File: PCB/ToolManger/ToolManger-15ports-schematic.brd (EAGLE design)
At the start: 187.9 x 114.9 mm, 52 parts, among them IC3 4049N, IC4 4049N, IC5 4049N

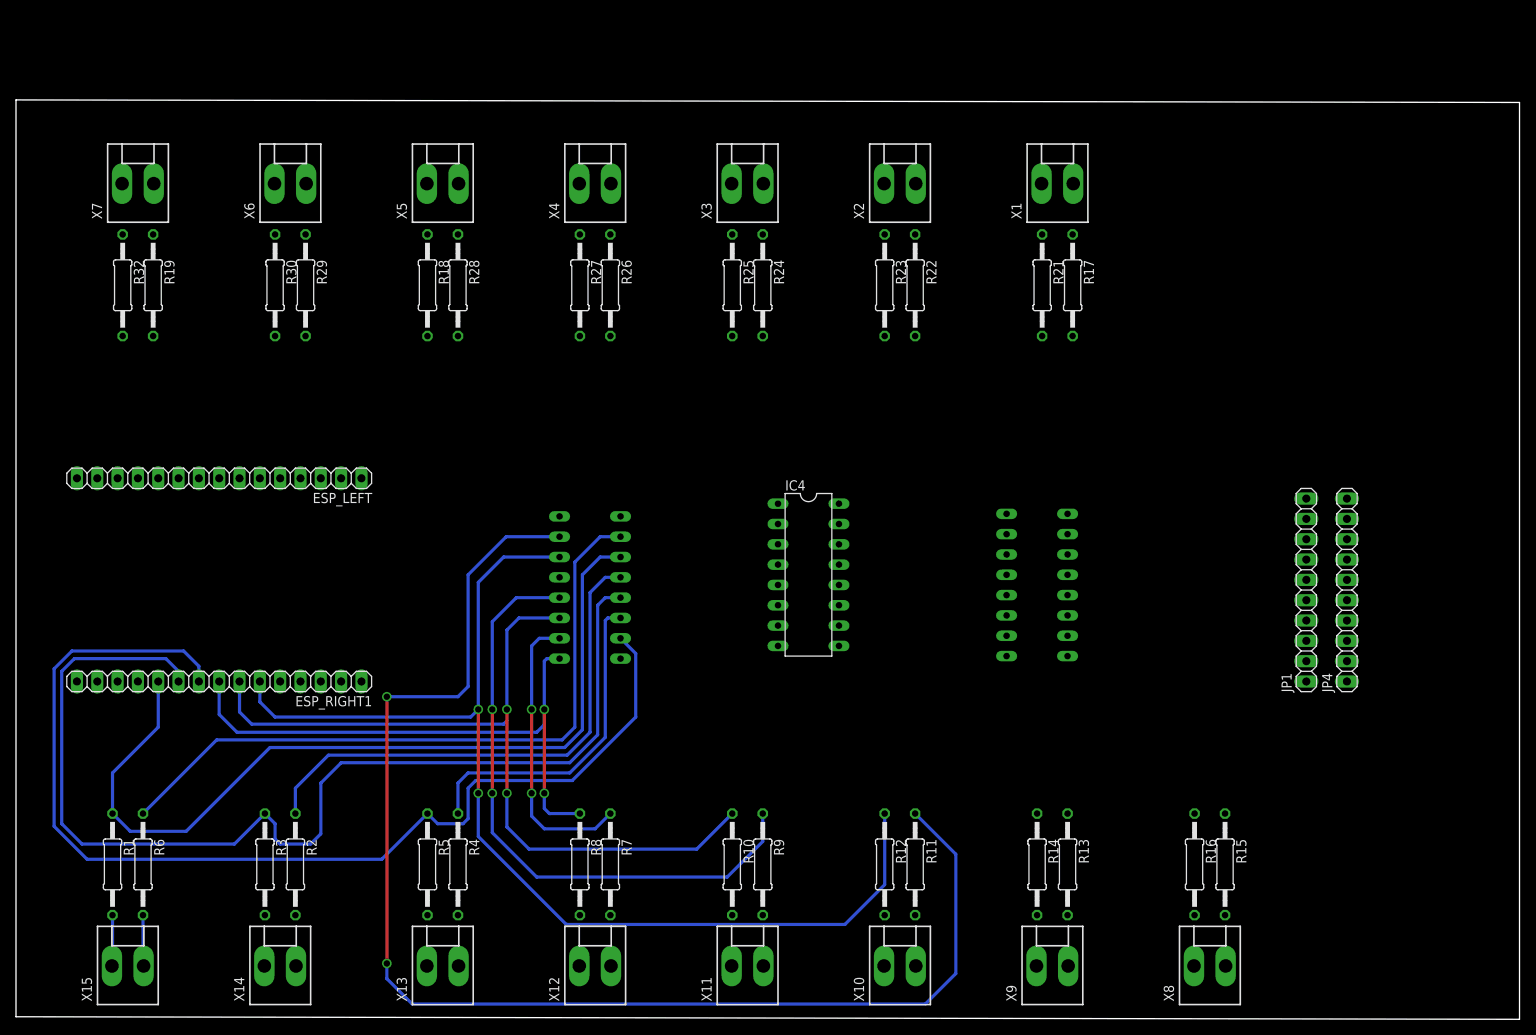
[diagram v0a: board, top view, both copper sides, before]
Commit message: UPDATE: board prototype finished
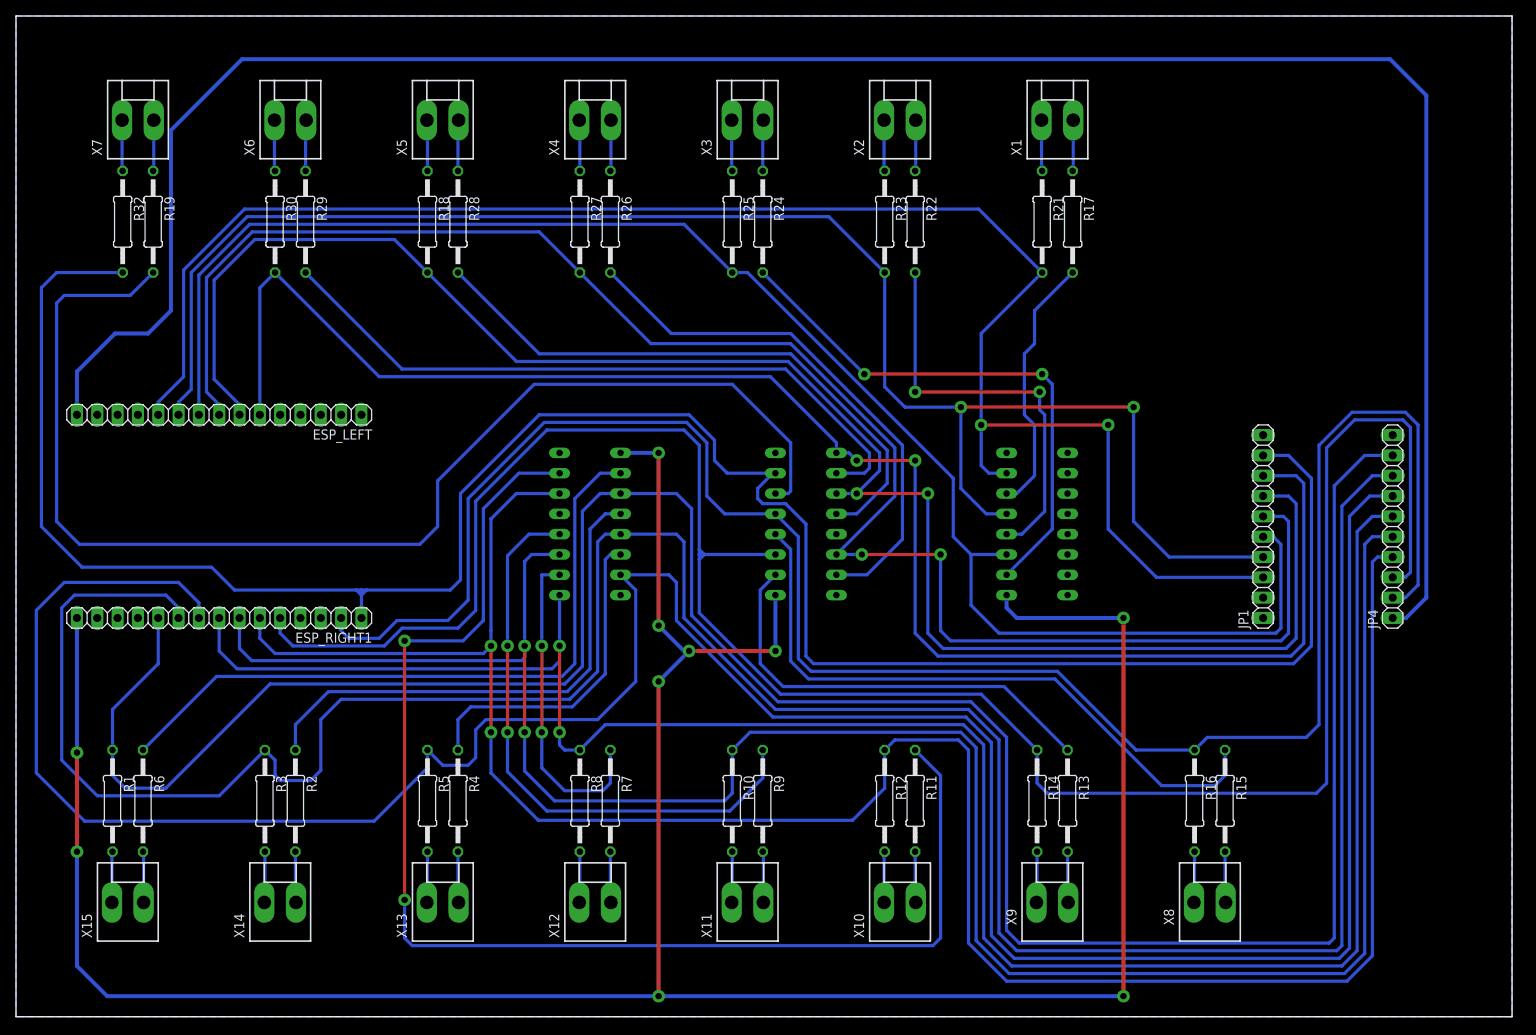
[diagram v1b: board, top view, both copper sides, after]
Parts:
- moved JP4 9.78 mm to (172.1, 61.3)
- moved JP1 9.60 mm to (155.9, 61.3)
- moved ESP_LEFT 7.94 mm to (25.4, 75.2)
- moved ESP_RIGHT1 7.94 mm to (25.4, 49.8)
- moved IC3 7.94 mm to (71.8, 61.6)
- moved R1 7.94 mm to (12.1, 27.0)
- moved R10 7.94 mm to (89.5, 27.0)
- moved R11 7.94 mm to (112.4, 27.0)
- moved R12 7.94 mm to (108.6, 27.0)
- moved R13 7.94 mm to (131.4, 27.0)
- moved R14 7.94 mm to (127.6, 27.0)
- moved R15 7.94 mm to (151.1, 27.0)
- moved R16 7.94 mm to (147.3, 27.0)
- moved R17 7.94 mm to (132.1, 99.4)
- moved R18 7.94 mm to (51.4, 99.4)
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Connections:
- new net +5V: ESP_LEFT.15, JP4.1
- net GND: now also ESP_LEFT.14, JP1.10
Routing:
- net +3V3: track 0.00 -> 333.9 mm, vias 0 -> 10
- net N$41: track 0.00 -> 281.8 mm
- net +5V: track 0.00 -> 273.4 mm
- net N$36: track 0.00 -> 272.7 mm
- net N$35: track 0.00 -> 247.5 mm
- net N$4: track 0.00 -> 218.3 mm, vias 0 -> 2
- net N$37: track 0.00 -> 218.1 mm, vias 0 -> 2
- net N$40: track 0.00 -> 214.8 mm, vias 0 -> 2
- net N$39: track 0.00 -> 206.9 mm, vias 0 -> 2
- net N$1: track 0.00 -> 206.5 mm, vias 0 -> 2
- net N$27: track 108.8 -> 312.9 mm
- net N$38: track 0.00 -> 202.3 mm
- net N$29: track 137.1 -> 337.6 mm
- net N$10: track 137.4 -> 333.5 mm
- net N$30: track 73.5 -> 254.9 mm
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- added copper zone on layer 16, net GND
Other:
- board size 187.9 x 114.9 mm -> 187 x 125.1 mm
